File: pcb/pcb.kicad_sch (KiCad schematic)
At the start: 24 parts

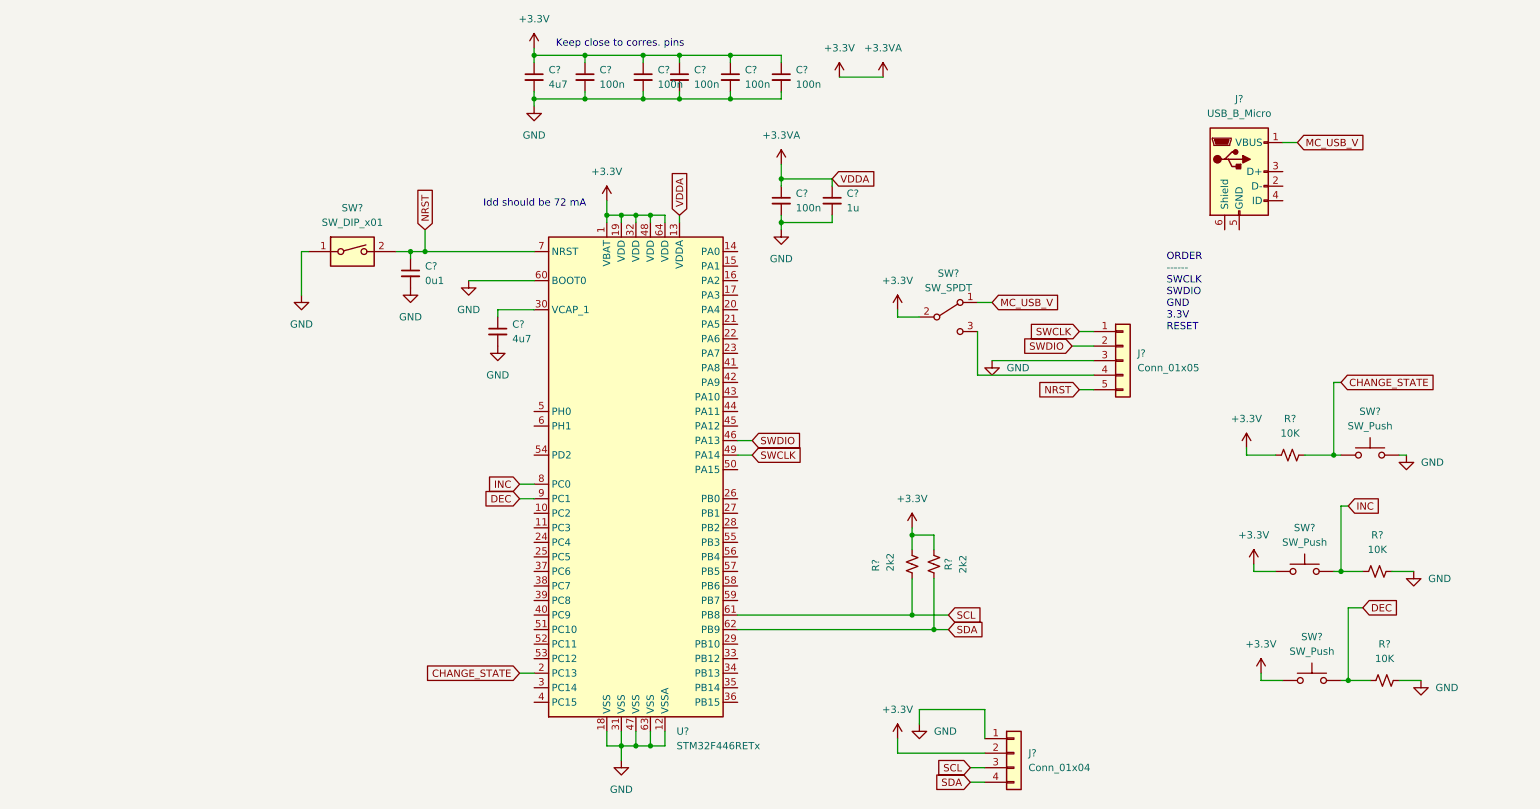
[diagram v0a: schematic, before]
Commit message: renamed stuff
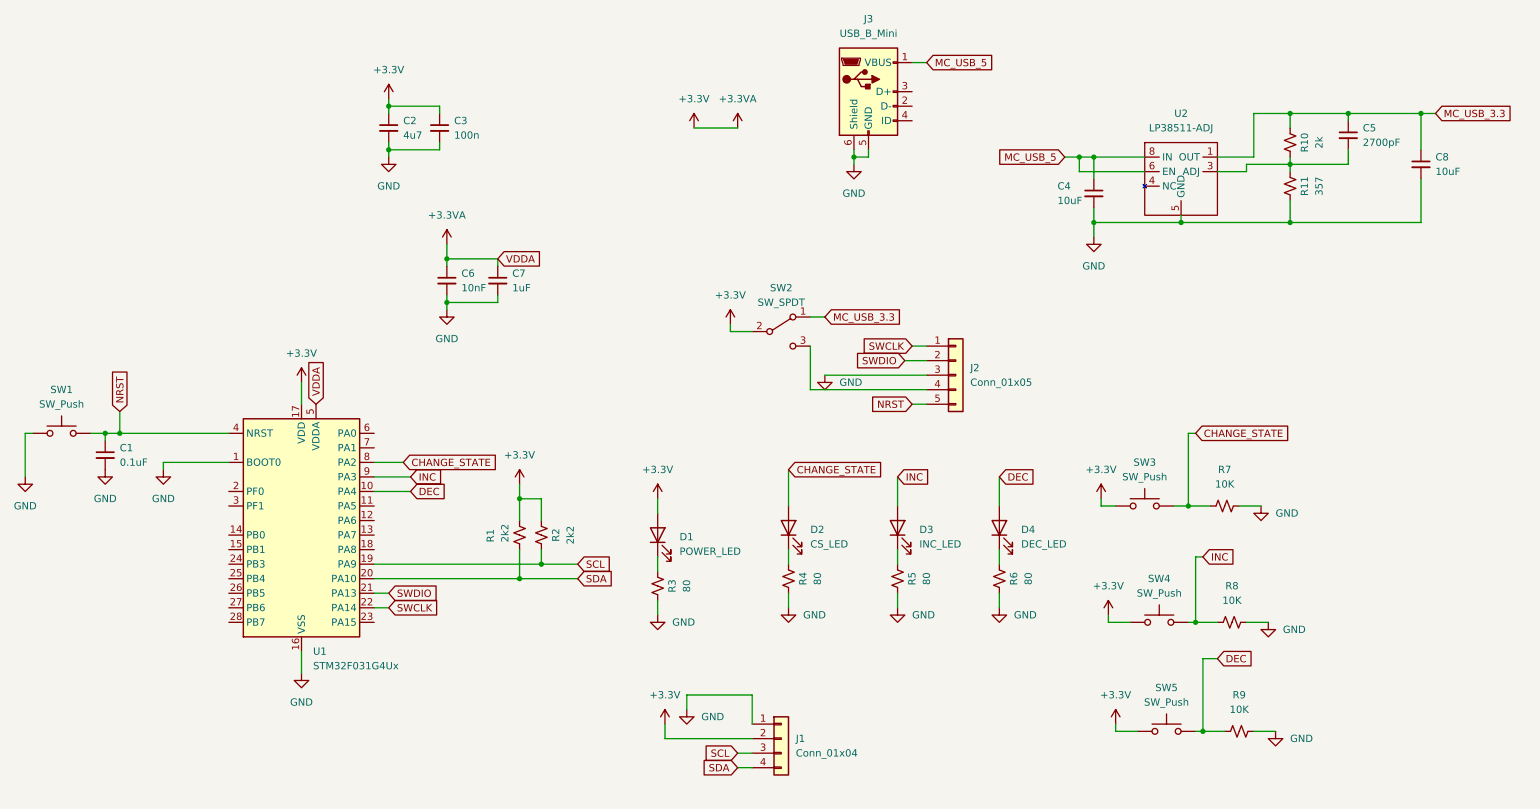
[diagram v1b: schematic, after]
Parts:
- removed C? (x6): 100n, symbol Device:C_Small
- removed C? (x2): 4u7, symbol Device:C_Small
- removed C?: 0u1, symbol Device:C_Small
- removed C?: 1u, symbol Device:C_Small
- removed J?: Conn_01x05, symbol Connector_Generic:Conn_01x05
- removed J?: Conn_01x04, symbol Connector_Generic:Conn_01x04
- removed J?: USB_B_Micro, symbol Connector:USB_B_Micro
- removed R? (x3): 10K, symbol Device:R_Small_US
- removed R? (x2): 2k2, symbol Device:R_Small_US
- removed SW? (x3): SW_Push, symbol Switch:SW_Push
- removed SW?: SW_SPDT, symbol Switch:SW_SPDT
- removed SW?: SW_DIP_x01, symbol Switch:SW_DIP_x01
- removed U?: STM32F446RETx, Package_QFP:LQFP-64_10x10mm_P0.5mm, symbol MCU_ST_STM32F4:STM32F446RETx
- added C1: 0.1uF, Capacitor_SMD:C_0805_2012Metric_Pad1.18x1.45mm_HandSolder, symbol Device:C_Small
- added C2: 4u7, Capacitor_SMD:C_0805_2012Metric_Pad1.18x1.45mm_HandSolder, symbol Device:C_Small
- added C3: 100n, Capacitor_SMD:C_0805_2012Metric_Pad1.18x1.45mm_HandSolder, symbol Device:C_Small
- added C4, C8: 10uF, Capacitor_SMD:C_0805_2012Metric_Pad1.18x1.45mm_HandSolder, symbol Device:C_Small
- added C5: 2700pF, Capacitor_SMD:C_0805_2012Metric_Pad1.18x1.45mm_HandSolder, symbol Device:C_Small
- added C6: 10nF, Capacitor_SMD:C_0805_2012Metric_Pad1.18x1.45mm_HandSolder, symbol Device:C_Small
- added C7: 1uF, Capacitor_SMD:C_0805_2012Metric_Pad1.18x1.45mm_HandSolder, symbol Device:C_Small
- added D1: POWER_LED, Diode_SMD:D_0805_2012Metric_Pad1.15x1.40mm_HandSolder, symbol Device:LED
- added D2: CS_LED, Diode_SMD:D_0805_2012Metric_Pad1.15x1.40mm_HandSolder, symbol Device:LED
- added D3: INC_LED, Diode_SMD:D_0805_2012Metric_Pad1.15x1.40mm_HandSolder, symbol Device:LED
- added D4: DEC_LED, Diode_SMD:D_0805_2012Metric_Pad1.15x1.40mm_HandSolder, symbol Device:LED
- added J1: Conn_01x04, Connector_PinSocket_2.54mm:PinSocket_1x04_P2.54mm_Vertical, symbol Connector_Generic:Conn_01x04
- added J2: Conn_01x05, Connector_PinHeader_2.54mm:PinHeader_1x05_P2.54mm_Vertical, symbol Connector_Generic:Conn_01x05
- added J3: USB_B_Mini, Connector_USB:USB_Mini-B_Lumberg_2486_01_Horizontal, symbol Connector:USB_B_Micro
- added R1, R2: 2k2, Resistor_SMD:R_0805_2012Metric_Pad1.20x1.40mm_HandSolder, symbol Device:R_Small_US
- added R10: 2k, Resistor_SMD:R_0805_2012Metric_Pad1.20x1.40mm_HandSolder, symbol Device:R_Small_US
- added R11: 357, Resistor_SMD:R_0805_2012Metric_Pad1.20x1.40mm_HandSolder, symbol Device:R_Small_US
- added R3, R4, R5, R6: 80, Resistor_SMD:R_0805_2012Metric_Pad1.20x1.40mm_HandSolder, symbol Device:R_Small_US
- added R7, R8, R9: 10K, Resistor_SMD:R_0805_2012Metric_Pad1.20x1.40mm_HandSolder, symbol Device:R_Small_US
- added SW1, SW3, SW4, SW5: SW_Push, MyLibrary:FSMSMTR-Tactile-Switch-FP, symbol Switch:SW_Push
- added SW2: SW_SPDT, MyLibrary:CL-SB-22A-01T-Slide-Switch-FP, symbol Switch:SW_SPDT
- added U1: STM32F031G4Ux, Package_DFN_QFN:QFN-28_4x4mm_P0.5mm, symbol MCU_ST_STM32F0:STM32F031G4Ux
- added U2: LP38511-ADJ, MyLibrary:TI_SO-PowerPAD-8-GND_DAP, symbol New_Library:LP38511-ADJ
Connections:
- net +3.3VA: now also C2.1, C3.1, C6.1, C7.1, D1.2 (A), J1.2 (Pin_2), R1.2, R2.2, SW2.2 (B), SW3.1, SW4.1, SW5.1, U1.17 (VDD), U1.5 (VDDA)
- net CHANGE_STATE: now also D2.2 (A), R7.1, SW3.2, U1.8 (PA2)
- net DEC: now also D4.2 (A), R9.1, SW5.2, U1.10 (PA4)
- net GND: now also C1.2, C2.2, C3.2, C4.2, C6.2, C7.2, C8.2, J1.1 (Pin_1), J2.3 (Pin_3), J3.5 (GND), J3.6 (Shield), R11.1, R3.1, R4.1, R5.1, R6.1, R7.2, R8.2, R9.2, SW1.1, U1.1 (BOOT0), U1.16 (VSS), U2.5 (GND)
- net INC: now also D3.2 (A), R8.1, SW4.2, U1.9 (PA3)
- net NRST: now also C1.1, J2.5 (Pin_5), SW1.2, U1.4 (NRST)
- net SCL: now also J1.3 (Pin_3), R2.1, U1.19 (PA9)
- net SDA: now also J1.4 (Pin_4), R1.1, U1.20 (PA10)
- net SWCLK: now also J2.1 (Pin_1), U1.22 (PA14)
- net SWDIO: now also J2.2 (Pin_2), U1.21 (PA13)
- new net: D4.1 (K), R6.2
- new net: C5.2, R10.1, R11.2, U2.3 (ADJ)
- new net: D3.1 (K), R5.2
- new net: J2.4 (Pin_4), SW2.3 (C)
- new net: D2.1 (K), R4.2
- new net: D1.1 (K), R3.2
- new net MC_USB_3.3: C5.1, C8.1, R10.2, SW2.1 (A), U2.1 (OUT)
- new net MC_USB_5: C4.1, J3.1 (VBUS), U2.6 (EN), U2.8 (IN)
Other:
- note removed: "Idd should be 72 mA"
- note removed: "Keep close to corres. pins"
- note removed: "ORDER ------ SWCLK SWDIO GND 3.3V RESET"
